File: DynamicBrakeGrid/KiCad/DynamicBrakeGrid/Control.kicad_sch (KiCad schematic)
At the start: 47 parts, among them IC1 ISO1042BDWVR, IC5 LM358DR, IC6 MCP2515-e_ST, Y1 8MHz

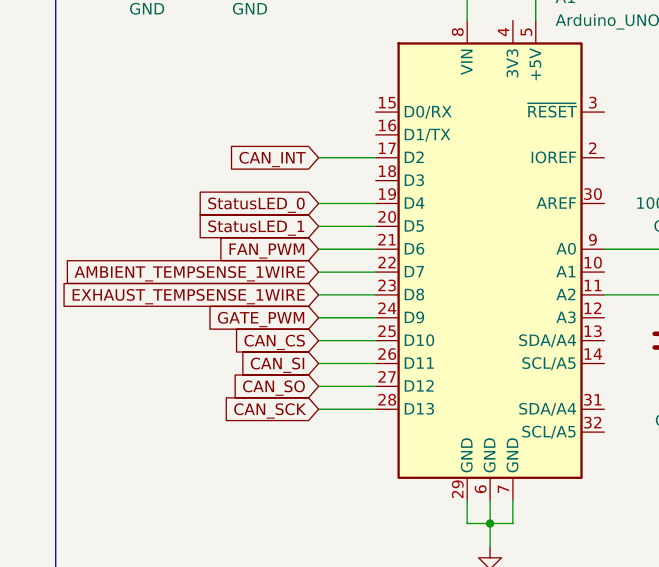
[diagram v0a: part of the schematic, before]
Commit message: u
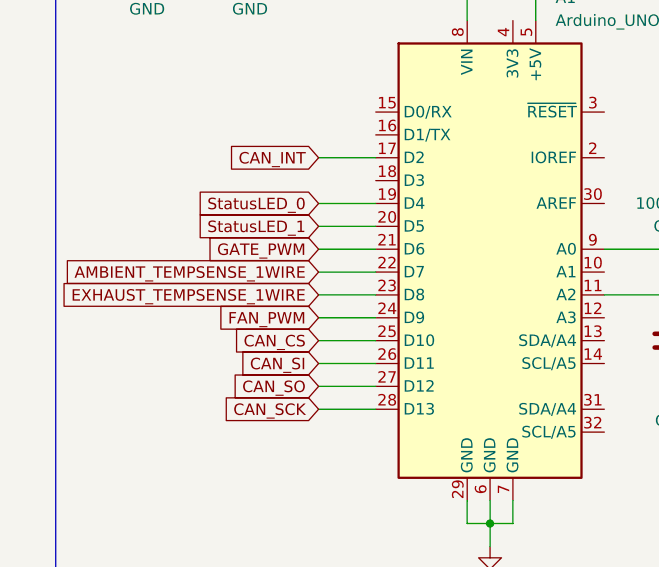
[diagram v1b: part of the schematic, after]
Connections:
- net FAN_PWM: now also A1.24 (D9); no longer A1.21 (D6)
- net GATE_PWM: now also A1.21 (D6); no longer A1.24 (D9)
